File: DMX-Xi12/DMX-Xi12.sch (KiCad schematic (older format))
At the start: 0 parts

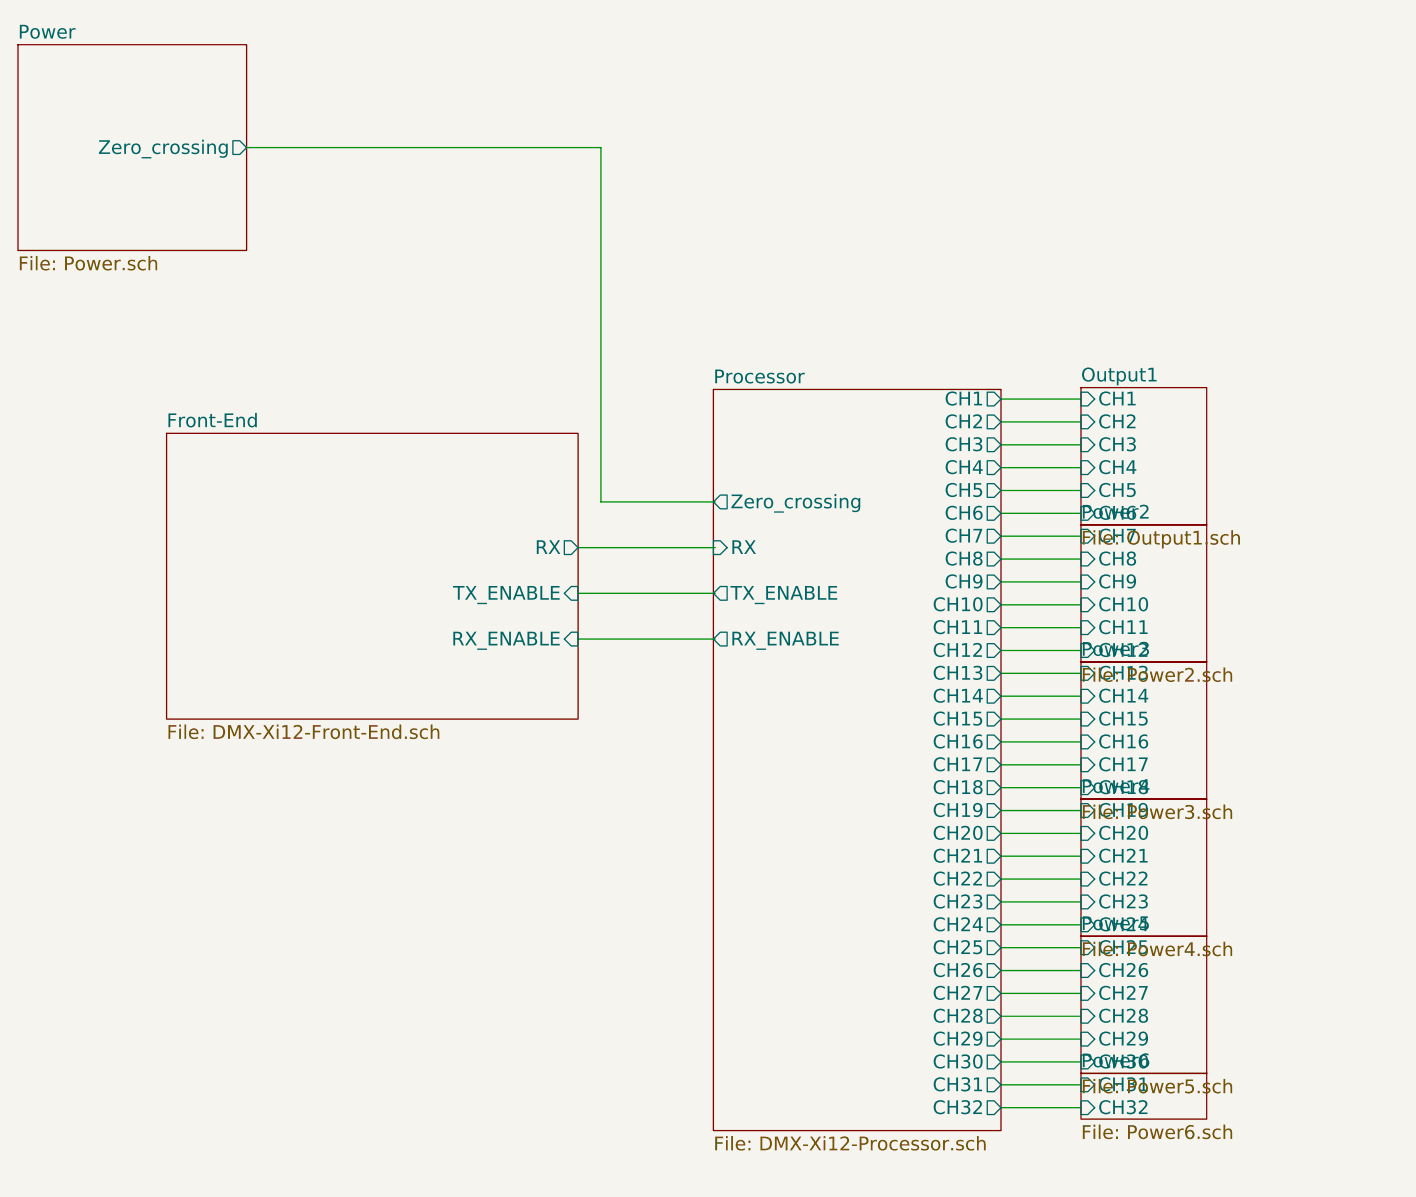
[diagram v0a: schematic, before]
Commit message: made dlaw changes etc
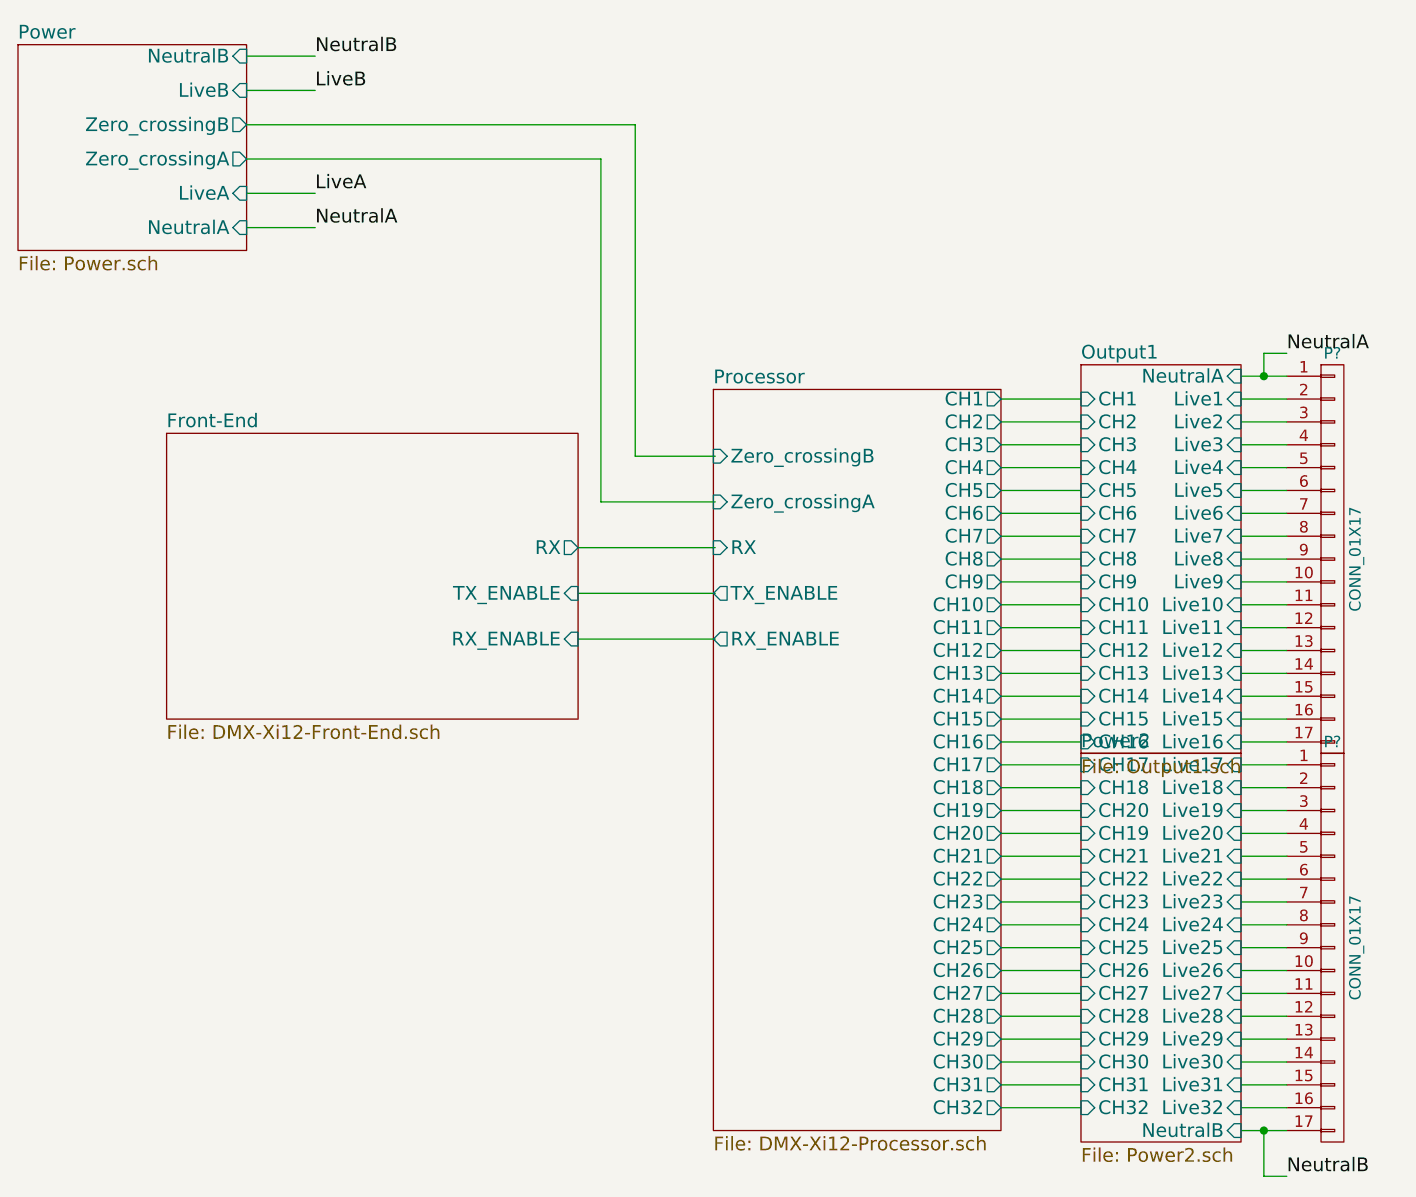
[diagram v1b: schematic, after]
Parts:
- added P? (x2): CONN_01X17, symbol CONN_01X17
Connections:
- net labels added: LiveA, LiveB, NeutralA, NeutralB
- wire segments 38 -> 83
